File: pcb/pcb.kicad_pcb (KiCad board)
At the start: 2 copper layers, 185.3 x 78.2 mm, 22 parts, among them J1 USB_C_Receptacle, J2 Conn_01x10_Pin, J3 Conn_01x10_Pin, J4 Conn_01x10_Pin, J5 Conn_01x10_Pin, J6 Conn_01x02_Pin, SW1 SW_Push, U1 W65C02SxP, U10 74HC04, U2 W65C22SxP, U3 W65C22SxP, U4 28C256, U5 HM62256BLP, U6 74HC684, U7 74HC680, U8 74HC680, U9 74HC00, Y1 MCO-1510A

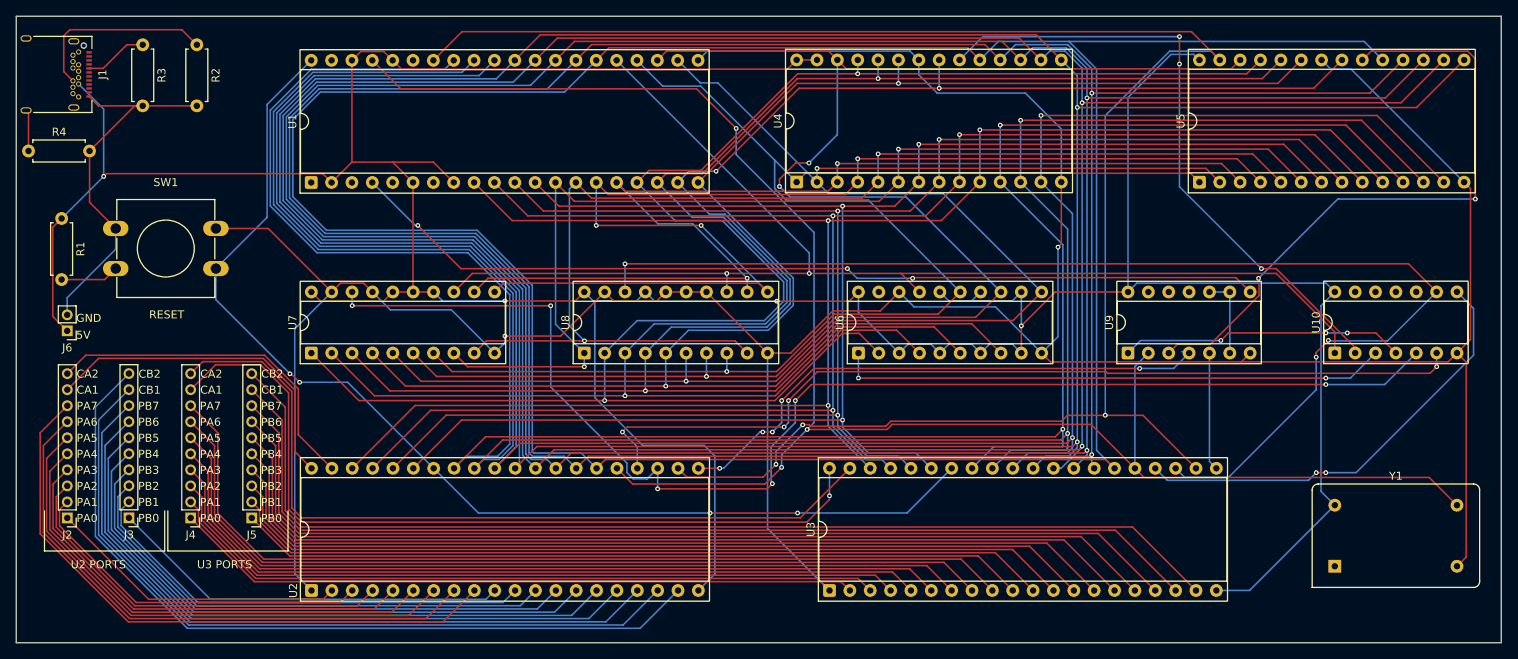
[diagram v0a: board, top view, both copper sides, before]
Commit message: update
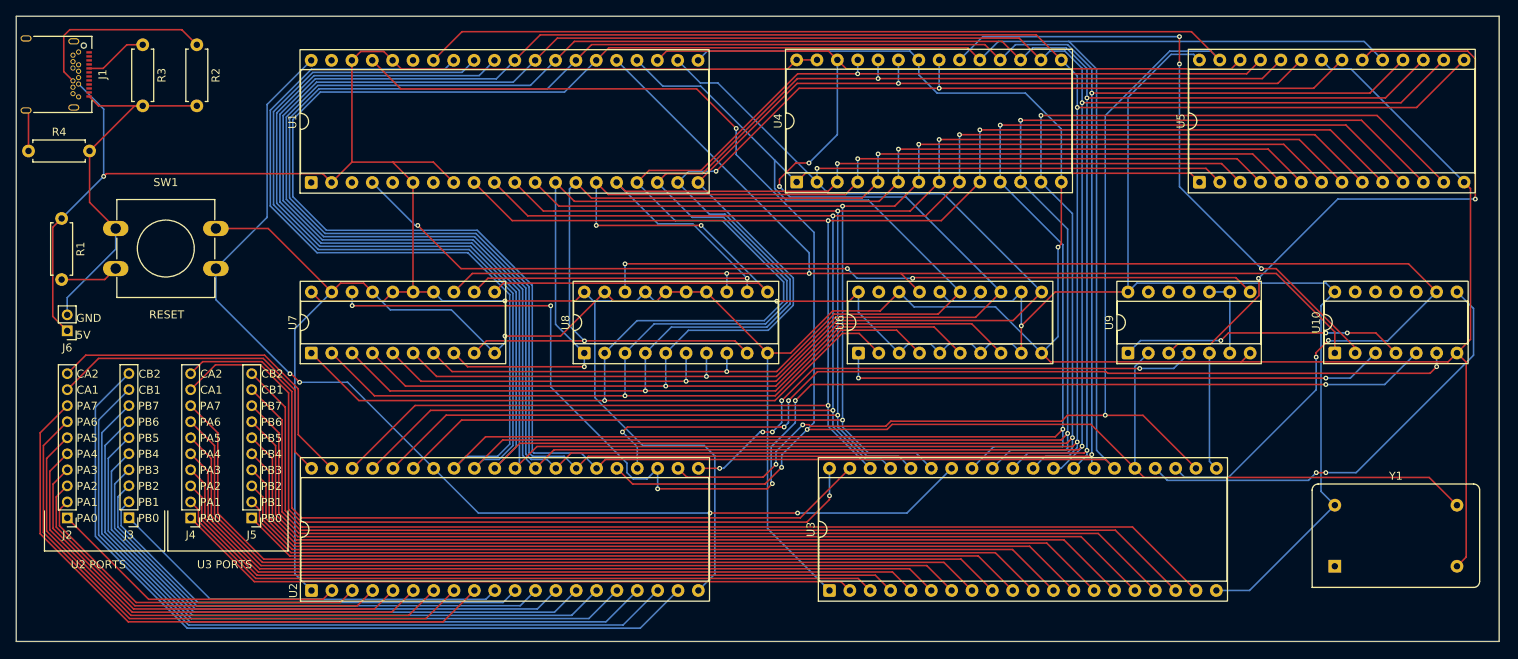
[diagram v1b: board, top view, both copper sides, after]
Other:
- board size 185.3 x 78.2 mm -> 185 x 78 mm
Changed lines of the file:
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@@
 			(drillshape 0)
 			(scaleselection 1)
-			(outputdirectory "")
+			(outputdirectory "Fabrication/")
 		)
 	)
@@
 	(gr_rect
 		(start 62.48 29.04)
-		(end 247.75 107.2)
+		(end 247.48 107.04)
 		(stroke
 			(width 0.05)

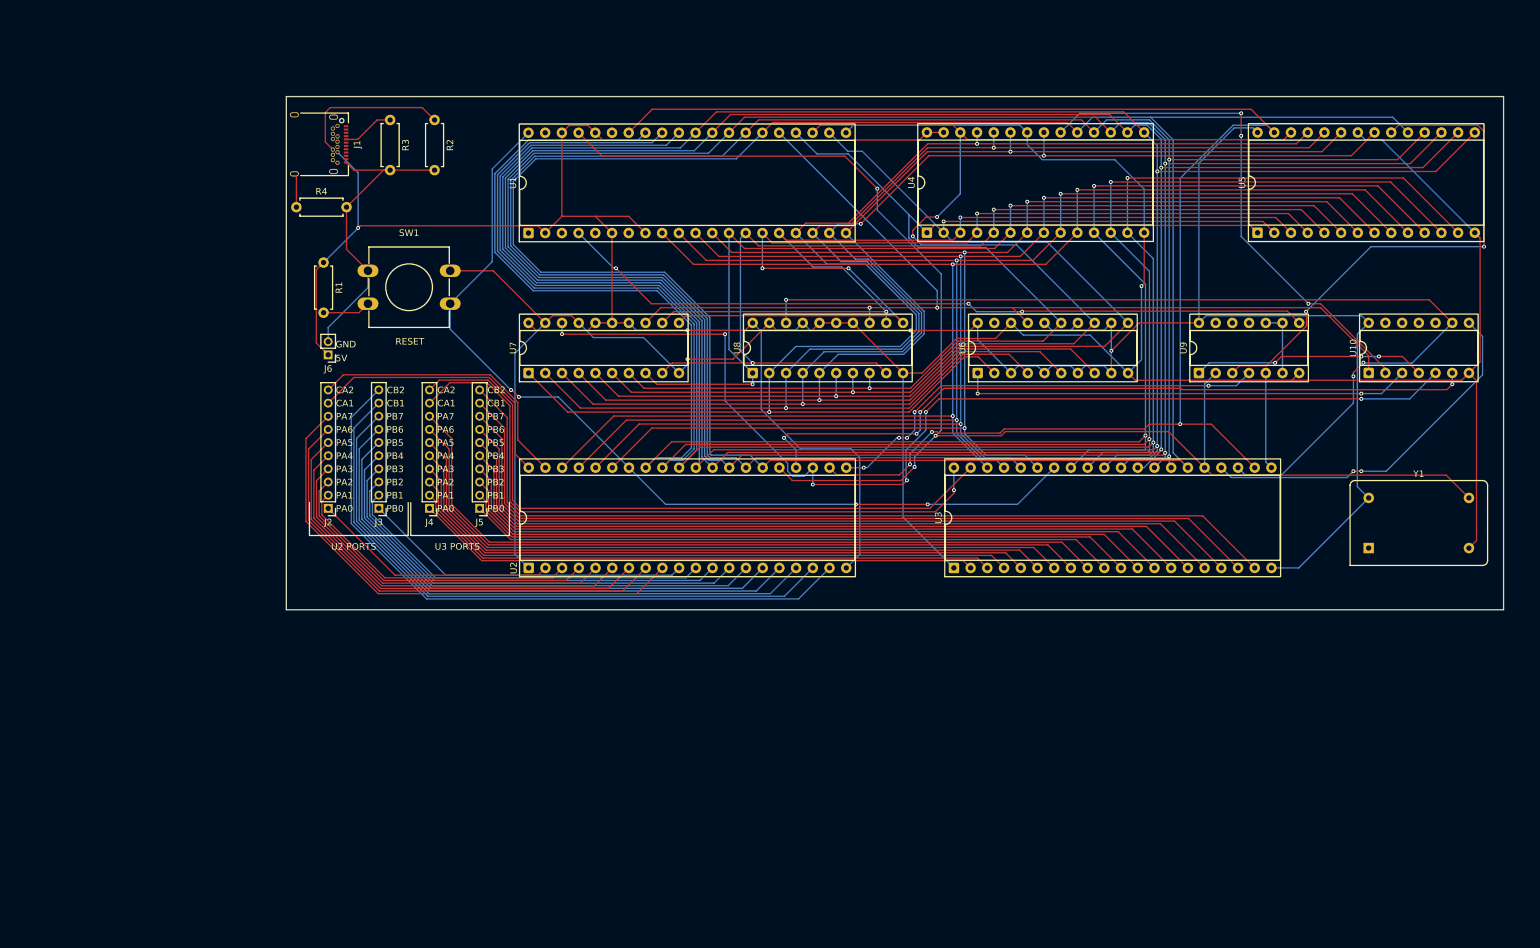
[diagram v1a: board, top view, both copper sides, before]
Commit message: Finished vesrsion 1 of the project
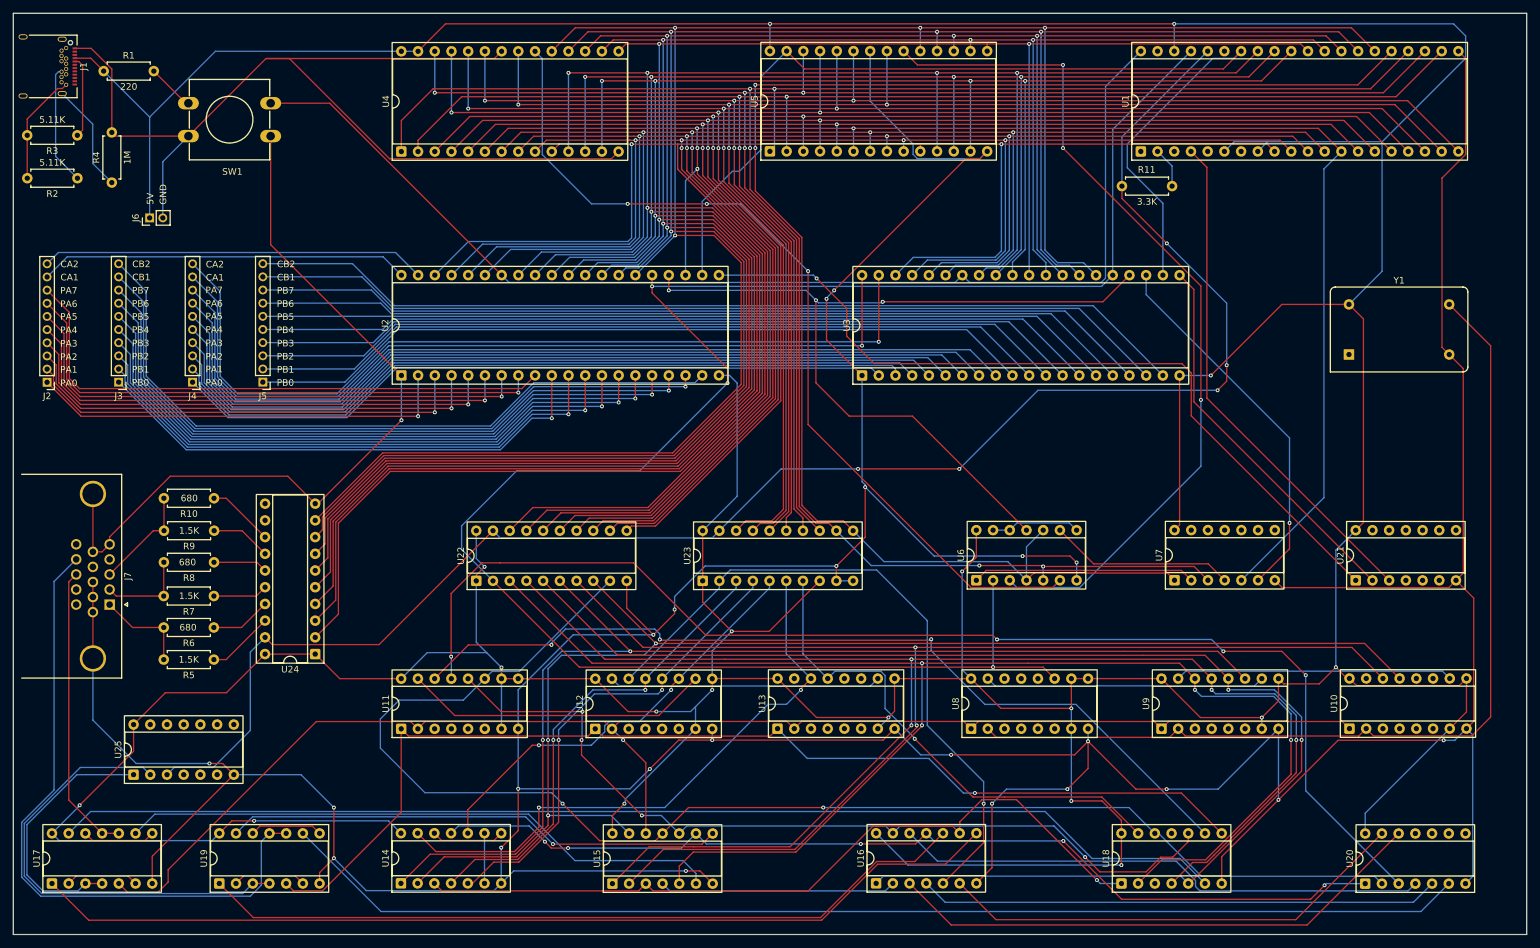
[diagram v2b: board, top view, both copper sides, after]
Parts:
- added J7: DE15_Socket_HighDensity_MountingHoles, Connector_Dsub:DSUB-15-HD_Socket_Horizontal_P2.29x2.54mm_EdgePinOffset8.35mm_Housed_MountingHolesOffset10.89mm, F.Cu at (35.6, 106.2)
- added R10: 680, Resistor_THT:R_Axial_DIN0207_L6.3mm_D2.5mm_P7.62mm_Horizontal, F.Cu at (51.5, 90.1)
- added R11: 3.3K, Resistor_THT:R_Axial_DIN0207_L6.3mm_D2.5mm_P7.62mm_Horizontal, F.Cu at (189.5, 42.6)
- added R5: 1.5K, Resistor_THT:R_Axial_DIN0207_L6.3mm_D2.5mm_P7.62mm_Horizontal, F.Cu at (51.5, 114.6)
- added R6: 680, Resistor_THT:R_Axial_DIN0207_L6.3mm_D2.5mm_P7.62mm_Horizontal, F.Cu at (51.5, 109.7)
- added R7: 1.5K, Resistor_THT:R_Axial_DIN0207_L6.3mm_D2.5mm_P7.62mm_Horizontal, F.Cu at (51.5, 105.0)
- added R8: 680, Resistor_THT:R_Axial_DIN0207_L6.3mm_D2.5mm_P7.62mm_Horizontal, F.Cu at (51.5, 99.8)
- added R9: 1.5K, Resistor_THT:R_Axial_DIN0207_L6.3mm_D2.5mm_P7.62mm_Horizontal, F.Cu at (51.5, 95.0)
- added U11: 74HC161, Package_DIP:DIP-16_W7.62mm_Socket, F.Cu at (79.9, 125.1)
- added U12: 74HC161, Package_DIP:DIP-16_W7.62mm_Socket, F.Cu at (109.4, 125.1)
- added U13: 74HC161, Package_DIP:DIP-16_W7.62mm_Socket, F.Cu at (137.1, 125.1)
- added U14: 74LS08, Package_DIP:DIP-14_W7.62mm_Socket, F.Cu at (79.9, 148.6)
- added U15: 74LS10, Package_DIP:DIP-14_W7.62mm_Socket, F.Cu at (112.0, 148.7)
- added U16: 74LS04, Package_DIP:DIP-14_W7.62mm_Socket, F.Cu at (152.1, 148.6)
- added U17: 74LS00, Package_DIP:DIP-14_W7.62mm_Socket, F.Cu at (26.9, 148.6)
- added U18: 74LS20, Package_DIP:DIP-14_W7.62mm_Socket, F.Cu at (189.4, 148.6)
- added U19: 74LS00, Package_DIP:DIP-14_W7.62mm_Socket, F.Cu at (52.3, 148.6)
- added U20: 74LS10, Package_DIP:DIP-14_W7.62mm_Socket, F.Cu at (226.4, 148.7)
- added U21: 74LS08, Package_DIP:DIP-14_W7.62mm_Socket, F.Cu at (225.0, 102.6)
- added U22: 74LS245, Package_DIP:DIP-20_W7.62mm_Socket, F.Cu at (91.3, 102.6)
- added U23: 74LS245, Package_DIP:DIP-20_W7.62mm_Socket, F.Cu at (125.8, 102.6)
- added U24: 74LS245, Package_DIP:DIP-20_W7.62mm_Socket, F.Cu at (66.9, 113.8)
- added U25: 74LS32, Package_DIP:DIP-14_W7.62mm_Socket, F.Cu at (39.3, 132.1)
- U10: value 74HC04 -> 74HC161; footprint Package_DIP:DIP-14_W7.62mm_Socket -> Package_DIP:DIP-16_W7.62mm_Socket
- U6: value 74HC684 -> 74HC00; footprint Package_DIP:DIP-20_W7.62mm_Socket -> Package_DIP:DIP-14_W7.62mm_Socket
- U7: value 74HC680 -> 74HC04; footprint Package_DIP:DIP-20_W7.62mm_Socket -> Package_DIP:DIP-14_W7.62mm_Socket
- U8: value 74HC680 -> 74HC161; footprint Package_DIP:DIP-20_W7.62mm_Socket -> Package_DIP:DIP-16_W7.62mm_Socket
- U9: value 74HC00 -> 74HC161; footprint Package_DIP:DIP-14_W7.62mm_Socket -> Package_DIP:DIP-16_W7.62mm_Socket
- Y1: value MCO-1510A -> 25.175 Mhz
- moved U7 103.1 mm to (197.5, 102.5)
- moved U1 93.9 mm to (192.3, 37.4)
- moved U4 80.8 mm to (80.0, 37.4)
- moved U5 75.1 mm to (136.0, 37.4)
- moved U8 63.4 mm to (166.6, 125.1)
- moved R2 55.0 mm to (30.7, 41.5), turned to 180 degrees
- moved U9 54.4 mm to (195.5, 125.1)
- moved U10 54.1 mm to (224.1, 125.1)
- moved R3 47.6 mm to (30.7, 34.9), turned to 180 degrees
- moved J2 46.8 mm to (26.1, 72.5)
- moved R1 44.3 mm to (34.7, 25.2), turned to 0 degrees
- moved J3 43.9 mm to (37.0, 72.5)
- moved J1 42.9 mm to (25.3, 24.5)
- moved J4 40.8 mm to (48.2, 72.5)
- moved J5 38.1 mm to (58.9, 72.4)
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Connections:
- U1 pad 13: /A4 -> ~{CS}_{VIA A}
- U1 pad 2: +5V -> Net-(U1-RDY)
- U1 pad 36: +5V -> CPU/~{VGA}
- U1 pad 37: CLK -> Clock
- U10 pad 1: /A15 -> Net-(U10-~{MR})
- U10 pad 10: (no net) -> Net-(U10-CET)
- U10 pad 11: (no net) -> unconnected-(U10-Q3-Pad11)
- U10 pad 12: (no net) -> unconnected-(U10-Q2-Pad12)
- U10 pad 13: (no net) -> /Q9A
- U10 pad 14: +5V -> /Q8A
- U10 pad 2: Net-(U4-~{CS}) -> Net-(U10-CP)
- U10 pad 3: Net-(U6-~{P>Q}) -> unconnected-(U10-D0-Pad3)
- U10 pad 4: Net-(U10-Pad4) -> unconnected-(U10-D1-Pad4)
- U10 pad 5: Net-(U2-~{CS2}) -> unconnected-(U10-D2-Pad5)
- U10 pad 6: Net-(U2-CS1) -> unconnected-(U10-D3-Pad6)
- U10 pad 7: GND -> +5V
- U10 pad 8: Net-(U3-CS1) -> GND
- U10 pad 9: Net-(U3-~{CS2}) -> +5V
- U2 pad 23: Net-(U2-~{CS2}) -> ~{CS}_{VIA A}
- U2 pad 24: Net-(U2-CS1) -> VIA Enable
- U2 pad 25: CLK -> Clock
- U3 pad 23: Net-(U3-~{CS2}) -> ~{CS}_{VIA B}
- U3 pad 24: Net-(U3-CS1) -> VIA Enable
- U3 pad 25: CLK -> Clock
- U4 pad 20: Net-(U4-~{CS}) -> ~{CS}_{ROM}
- U4 pad 6: /A4 -> ~{CS}_{VIA A}
- U5 pad 20: Net-(U5-~{CS}) -> ~{CS}_{RAM}
- U5 pad 6: /A4 -> ~{CS}_{VIA A}
- U6 pad 1: Net-(U6-~{P>Q}) -> Net-(U6-Pad1)
- U6 pad 10: GND -> /A15
- U6 pad 11: /A12 -> VIA Enable
- U6 pad 12: +5V -> Net-(U6-Pad12)
- U6 pad 13: /A13 -> Net-(U6-Pad12)
- U6 pad 2: /A8 -> Clock
- U6 pad 3: +5V -> ~{CS}_{RAM}
- U6 pad 4: /A9 -> /A15
- U6 pad 5: +5V -> /A14
- U6 pad 6: /A10 -> ~{CS}_{ROM}
- U6 pad 7: +5V -> GND
- U6 pad 8: /A11 -> Net-(U6-Pad12)
- U6 pad 9: +5V -> Net-(U6-Pad9)
- U7 pad 1: /A8 -> /A15
- U7 pad 10: GND -> (no net)
- U7 pad 11: /A6 -> (no net)
- U7 pad 12: /A7 -> (no net)
- U7 pad 13: /A15 -> (no net)
- U7 pad 2: /A9 -> Net-(U6-Pad1)
- U7 pad 3: /A10 -> /A14
- U7 pad 4: /A11 -> Net-(U6-Pad9)
- U7 pad 5: /A12 -> ~{CS}_{VIA A}
- U7 pad 6: /A13 -> ~{CS}_{VIA B}
- U7 pad 7: /A14 -> GND
- U7 pad 8: /A4 -> (no net)
- U7 pad 9: /A5 -> (no net)
- U8 pad 1: /A4 -> Net-(U10-~{MR})
- U8 pad 10: GND -> +5V
- U8 pad 11: /A6 -> Clock
- U8 pad 12: /A7 -> unconnected-(U8-Q2-Pad12)
- U8 pad 13: /A15 -> unconnected-(U8-Q1-Pad13)
- U8 pad 14: GND -> unconnected-(U8-Q0-Pad14)
- U8 pad 15: GND -> Net-(U8-TC)
- U8 pad 16: GND -> +5V
- U8 pad 2: /A8 -> Net-(U10-CP)
- U8 pad 3: /A9 -> unconnected-(U8-D0-Pad3)
- U8 pad 4: /A10 -> unconnected-(U8-D1-Pad4)
- U8 pad 5: /A11 -> unconnected-(U8-D2-Pad5)
- U8 pad 6: /A12 -> unconnected-(U8-D3-Pad6)
- U8 pad 7: /A13 -> +5V
- U8 pad 8: /A14 -> GND
- U8 pad 9: /A5 -> +5V
- U9 pad 1: Net-(U10-Pad4) -> Net-(U10-~{MR})
- U9 pad 10: Net-(U9-Pad10) -> Net-(U8-TC)
- U9 pad 11: (no net) -> /Q7A
- U9 pad 12: (no net) -> /Q6A
- U9 pad 13: (no net) -> /Q5A
- U9 pad 14: +5V -> /Q4A
- U9 pad 2: CLK -> Net-(U10-CP)
- U9 pad 3: Net-(U5-~{CS}) -> unconnected-(U9-D0-Pad3)
- U9 pad 4: ~{IRQ} 1 -> unconnected-(U9-D1-Pad4)
- U9 pad 5: ~{IRQ} 2 -> unconnected-(U9-D2-Pad5)
- U9 pad 6: Net-(U9-Pad10) -> unconnected-(U9-D3-Pad6)
- U9 pad 7: GND -> +5V
- U9 pad 8: Net-(U1-~{IRQ}) -> GND
- U9 pad 9: Net-(U9-Pad10) -> +5V
- Y1 pad 8: CLK -> Net-(U10-CP)
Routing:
- net GND: track 452.8 -> 1090.3 mm, vias 2 -> 24
- net +5V: track 463.9 -> 1000.6 mm, vias 4 -> 18
- net ~{CS}_{VIA A}: track 0.00 -> 308.9 mm, vias 0 -> 4
- net Clock: track 0.00 -> 295.3 mm, vias 0 -> 3
- net CPU/~{VGA}: track 0.00 -> 256.8 mm, vias 0 -> 5
- net /Q5A: track 0.00 -> 226.6 mm, vias 0 -> 4
- net /Q4A: track 0.00 -> 225.2 mm, vias 0 -> 4
- net Net-(U10-~{MR}): track 0.00 -> 222.5 mm, vias 0 -> 1
- net CLK: track 219.7 -> 0.00 mm, vias 3 -> 0
- net /Q3B: track 0.00 -> 212.9 mm, vias 0 -> 2
- net /Q9A: track 0.00 -> 207.4 mm, vias 0 -> 3
- net /Q6A: track 0.00 -> 205.7 mm, vias 0 -> 2
- net /Q8A: track 0.00 -> 194.5 mm, vias 0 -> 2
- net /Q1B: track 0.00 -> 189.4 mm, vias 0 -> 4
- net Net-(U19-Pad9): track 0.00 -> 180.8 mm
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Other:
- board size 185 x 78 mm -> 230 x 140 mm
- board text removed: "RESET"
- board text removed: "U2 PORTS"
- board text removed: "U3 PORTS"

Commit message: started working on version 2.0
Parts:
- removed J4, J5: Conn_01x10_Pin, Connector_PinHeader_2.00mm:PinHeader_1x10_P2.00mm_Vertical
- removed J6: Conn_01x02_Pin, Connector_PinHeader_2.00mm:PinHeader_1x02_P2.00mm_Vertical
- removed J7: DE15_Socket_HighDensity_MountingHoles, Connector_Dsub:DSUB-15-HD_Socket_Horizontal_P2.29x2.54mm_EdgePinOffset8.35mm_Housed_MountingHolesOffset10.89mm
- removed R10, R8: 680, Resistor_THT:R_Axial_DIN0207_L6.3mm_D2.5mm_P7.62mm_Horizontal
- removed R11: 3.3K, Resistor_THT:R_Axial_DIN0207_L6.3mm_D2.5mm_P7.62mm_Horizontal
- removed R9: 1.5K, Resistor_THT:R_Axial_DIN0207_L6.3mm_D2.5mm_P7.62mm_Horizontal
- removed U10, U11, U12, U13: 74HC161, Package_DIP:DIP-16_W7.62mm_Socket
- removed U14, U21: 74LS08, Package_DIP:DIP-14_W7.62mm_Socket
- removed U15, U20: 74LS10, Package_DIP:DIP-14_W7.62mm_Socket
- removed U16: 74LS04, Package_DIP:DIP-14_W7.62mm_Socket
- removed U17, U19: 74LS00, Package_DIP:DIP-14_W7.62mm_Socket
- removed U18: 74LS20, Package_DIP:DIP-14_W7.62mm_Socket
- removed U22, U23, U24: 74LS245, Package_DIP:DIP-20_W7.62mm_Socket
- removed U25: 74LS32, Package_DIP:DIP-14_W7.62mm_Socket
- removed Y1: 25.175 Mhz, Oscillator:Oscillator_DIP-14
- added C1: 100nF, Capacitor_SMD:C_0805_2012Metric_Pad1.18x1.45mm_HandSolder, B.Cu at (87.1, 47.8)
- added C2: 100nF, Capacitor_SMD:C_0805_2012Metric_Pad1.18x1.45mm_HandSolder, B.Cu at (169.8, 33.9)
- added C3: 100nF, Capacitor_SMD:C_0805_2012Metric_Pad1.18x1.45mm_HandSolder, B.Cu at (125.3, 37.6)
- added C4: 100nF, Capacitor_SMD:C_0805_2012Metric_Pad1.18x1.45mm_HandSolder, F.Cu at (117.8, 79.1)
- added C5: 100nF, Capacitor_SMD:C_0805_2012Metric_Pad1.18x1.45mm_HandSolder, F.Cu at (172.2, 79.1)
- added C6: 100nF, Capacitor_SMD:C_0805_2012Metric_Pad1.18x1.45mm_HandSolder, B.Cu at (56.0, 39.0)
- added C7: 100nF, Capacitor_SMD:C_0805_2012Metric_Pad1.18x1.45mm_HandSolder, F.Cu at (62.0, 32.8)
- J2, J3: value Conn_01x10_Pin -> 2x20 Header; footprint Connector_PinHeader_2.00mm:PinHeader_1x10_P2.00mm_Vertical -> Connector_PinHeader_2.54mm:PinHeader_2x10_P2.54mm_Vertical
- R1: value 220 -> 1M; footprint Resistor_THT:R_Axial_DIN0207_L6.3mm_D2.5mm_P7.62mm_Horizontal -> Resistor_SMD:R_0805_2012Metric_Pad1.20x1.40mm_HandSolder
- R2, R3: value 5.11K -> 5K1; footprint Resistor_THT:R_Axial_DIN0207_L6.3mm_D2.5mm_P7.62mm_Horizontal -> Resistor_SMD:R_0805_2012Metric_Pad1.20x1.40mm_HandSolder
- R4: value 1M -> 3K3; footprint Resistor_THT:R_Axial_DIN0207_L6.3mm_D2.5mm_P7.62mm_Horizontal -> Resistor_SMD:R_0805_2012Metric_Pad1.20x1.40mm_HandSolder; moved to B.Cu
- R5: value 1.5K -> 10K; footprint Resistor_THT:R_Axial_DIN0207_L6.3mm_D2.5mm_P7.62mm_Horizontal -> Resistor_SMD:R_0805_2012Metric_Pad1.20x1.40mm_HandSolder
- R6: value 680 -> 1M; footprint Resistor_THT:R_Axial_DIN0207_L6.3mm_D2.5mm_P7.62mm_Horizontal -> Resistor_SMD:R_0805_2012Metric_Pad1.20x1.40mm_HandSolder
- R7: value 1.5K -> 10K; footprint Resistor_THT:R_Axial_DIN0207_L6.3mm_D2.5mm_P7.62mm_Horizontal -> Resistor_SMD:R_0805_2012Metric_Pad1.20x1.40mm_HandSolder; moved to B.Cu
- SW1: footprint Button_Switch_THT:SW_PUSH-12mm -> Button_Switch_THT:SW_TH_Tactile_Omron_B3F-100x
- U1: value W65C02SxP -> W65C02
- U2: value W65C22SxP -> 28C256; footprint Package_DIP:DIP-40_W15.24mm_Socket -> Socket:DIP_Socket-28_W11.9mm_W12.7mm_W15.24mm_W17.78mm_W18.5mm_3M_228-1277-00-0602J
- U3: value W65C22SxP -> 62256; footprint Package_DIP:DIP-40_W15.24mm_Socket -> Package_DIP:DIP-28_W15.24mm_Socket
- U4: value 28C256 -> W65C22S; footprint Package_DIP:DIP-28_W15.24mm_Socket -> Package_DIP:DIP-40_W15.24mm_Socket
- U5: value HM62256BLP -> W65C22S; footprint Package_DIP:DIP-28_W15.24mm_Socket -> Package_DIP:DIP-40_W15.24mm_Socket
- U6: value 74HC00 -> 74AC00
- U7: value 74HC04 -> 74LS04
- U8: value 74HC161 -> 74LS08; footprint Package_DIP:DIP-16_W7.62mm_Socket -> Package_DIP:DIP-14_W7.62mm_Socket
- U9: value 74HC161 -> 555; footprint Package_DIP:DIP-16_W7.62mm_Socket -> Package_DIP:DIP-8_W7.62mm
- moved U7 336.3 mm to (-132.4, 37.0), turned to 0 degrees
- moved U6 318.3 mm to (-144.1, 37.0), turned to 0 degrees
- moved U8 300.5 mm to (-120.7, 37.0), turned to 0 degrees
- moved U9 162.0 mm to (56.0, 42.8)
- moved U2 126.8 mm to (201.8, 36.4), turned to -90 degrees
- moved U1 122.7 mm to (70.3, 50.3)
- moved R5 82.7 mm to (42.0, 32.5), turned to -90 degrees
- moved R6 77.2 mm to (57.0, 32.8), turned to 0 degrees
- moved R7 64.8 mm to (82.0, 47.8), turned to 0 degrees
- moved U5 40.0 mm to (124.9, 75.8)
- moved U4 39.6 mm to (70.5, 75.8)
- moved R4 36.9 mm to (72.9, 42.7), turned to -90 degrees
- moved U3 33.2 mm to (124.3, 50.3)
- moved J3 25.0 mm to (52.8, 53.0), turned to 0 degrees
- moved J2 21.9 mm to (36.1, 53.0), turned to 0 degrees
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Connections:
- J2 pad 1: Net-(J2-Pin_1) -> Net-(U4-PA0)
- J2 pad 10: Net-(J2-Pin_10) -> Net-(U4-PB4)
- J2 pad 2: Net-(J2-Pin_2) -> Net-(U4-PB0)
- J2 pad 3: Net-(J2-Pin_3) -> Net-(U4-PA1)
- J2 pad 4: Net-(J2-Pin_4) -> Net-(U4-PB1)
- J2 pad 5: Net-(J2-Pin_5) -> Net-(U4-PA2)
- J2 pad 6: Net-(J2-Pin_6) -> Net-(U4-PB2)
- J2 pad 7: Net-(J2-Pin_7) -> Net-(U4-PA3)
- J2 pad 8: Net-(J2-Pin_8) -> Net-(U4-PB3)
- J2 pad 9: Net-(J2-Pin_9) -> Net-(U4-PA4)
- J3 pad 1: Net-(J3-Pin_1) -> Net-(U5-PA0)
- J3 pad 10: Net-(J3-Pin_10) -> Net-(U5-PB4)
- J3 pad 2: Net-(J3-Pin_2) -> Net-(U5-PB0)
- J3 pad 3: Net-(J3-Pin_3) -> Net-(U5-PA1)
- J3 pad 4: Net-(J3-Pin_4) -> Net-(U5-PB1)
- J3 pad 5: Net-(J3-Pin_5) -> Net-(U5-PA2)
- J3 pad 6: Net-(J3-Pin_6) -> Net-(U5-PB2)
- J3 pad 7: Net-(J3-Pin_7) -> Net-(U5-PA3)
- J3 pad 8: Net-(J3-Pin_8) -> Net-(U5-PB3)
- J3 pad 9: Net-(J3-Pin_9) -> Net-(U5-PA4)
- R1 pad 1: +5V -> Net-(J1-SHIELD)
- R1 pad 2: ~{RES} -> GND
- R4 pad 1: Net-(J1-SHIELD) -> Net-(U1-BE)
- R4 pad 2: GND -> Net-(U1-RDY)
- R5 pad 1: Net-(U24-B0) -> +5V
- R5 pad 2: Net-(J7-Pad1) -> Net-(U9-TR)
- R6 pad 1: Net-(U24-B1) -> +5V
- R6 pad 2: Net-(J7-Pad1) -> Net-(U9-DIS)
- R7 pad 1: Net-(U24-B2) -> +5V
- R7 pad 2: Net-(J7-Pad2) -> ~{NMI}
- SW1 pad 2: ~{RES} -> Net-(U9-TR)
- U1 pad 13: ~{CS}_{VIA A} -> /A4
- U1 pad 36: CPU/~{VGA} -> Net-(U1-BE)
- U1 pad 37: Clock -> CLK
- U1 pad 4: Net-(U1-~{IRQ}) -> ~{IRQ}
- U1 pad 6: +5V -> ~{NMI}
- U2 pad 1: GND -> /A14
- U2 pad 10: Net-(J3-Pin_1) -> /A0
- U2 pad 11: Net-(J3-Pin_2) -> /D0
- U2 pad 12: Net-(J3-Pin_3) -> /D1
- U2 pad 13: Net-(J3-Pin_4) -> /D2
- U2 pad 14: Net-(J3-Pin_5) -> GND
- U2 pad 15: Net-(J3-Pin_6) -> /D3
- U2 pad 16: Net-(J3-Pin_7) -> /D4
- U2 pad 17: Net-(J3-Pin_8) -> /D5
- U2 pad 18: Net-(J3-Pin_9) -> /D6
- U2 pad 19: Net-(J3-Pin_10) -> /D7
- U2 pad 2: Net-(J2-Pin_1) -> /A12
- U2 pad 20: +5V -> unconnected-(U2-~{CS}-Pad20)
- U2 pad 21: ~{IRQ} 1 -> /A10
- U2 pad 22: R/~{W} -> GND
- U2 pad 23: ~{CS}_{VIA A} -> /A11
- U2 pad 24: VIA Enable -> /A9
- U2 pad 25: Clock -> /A8
- U2 pad 26: /D7 -> /A13
- U2 pad 27: /D6 -> GND
- U2 pad 28: /D5 -> +5V
- U2 pad 3: Net-(J2-Pin_2) -> /A7
- U2 pad 4: Net-(J2-Pin_3) -> /A6
- U2 pad 5: Net-(J2-Pin_4) -> /A5
- U2 pad 6: Net-(J2-Pin_5) -> /A4
- U2 pad 7: Net-(J2-Pin_6) -> /A3
- U2 pad 8: Net-(J2-Pin_7) -> /A2
- U2 pad 9: Net-(J2-Pin_8) -> /A1
- U3 pad 1: GND -> /A14
- U3 pad 10: Net-(J5-Pin_1) -> /A0
- U3 pad 11: Net-(J5-Pin_2) -> /D0
- U3 pad 12: Net-(J5-Pin_3) -> /D1
- U3 pad 13: Net-(J5-Pin_4) -> /D2
- U3 pad 14: Net-(J5-Pin_5) -> GND
- U3 pad 15: Net-(J5-Pin_6) -> /D3
- U3 pad 16: Net-(J5-Pin_7) -> /D4
- U3 pad 17: Net-(J5-Pin_8) -> /D5
- U3 pad 18: Net-(J5-Pin_9) -> /D6
- U3 pad 19: Net-(J5-Pin_10) -> /D7
- U3 pad 2: Net-(J4-Pin_1) -> /A12
- U3 pad 20: +5V -> unconnected-(U3-~{CS}-Pad20)
- U3 pad 21: ~{IRQ} 2 -> /A10
- U3 pad 22: R/~{W} -> GND
- U3 pad 23: ~{CS}_{VIA B} -> /A11
- U3 pad 24: VIA Enable -> /A9
- U3 pad 25: Clock -> /A8
- U3 pad 26: /D7 -> /A13
- U3 pad 27: /D6 -> R/~{W}
- U3 pad 28: /D5 -> +5V
- U3 pad 3: Net-(J4-Pin_2) -> /A7
- U3 pad 4: Net-(J4-Pin_3) -> /A6
- U3 pad 5: Net-(J4-Pin_4) -> /A5
- U3 pad 6: Net-(J4-Pin_5) -> /A4
- U3 pad 7: Net-(J4-Pin_6) -> /A3
- U3 pad 8: Net-(J4-Pin_7) -> /A2
- U3 pad 9: Net-(J4-Pin_8) -> /A1
- U4 pad 1: /A14 -> GND
- U4 pad 10: /A0 -> Net-(U4-PB0)
- U4 pad 11: /D0 -> Net-(U4-PB1)
- U4 pad 12: /D1 -> Net-(U4-PB2)
- U4 pad 13: /D2 -> Net-(U4-PB3)
- U4 pad 14: GND -> Net-(U4-PB4)
- U4 pad 15: /D3 -> Net-(U4-PB5)
- U4 pad 16: /D4 -> Net-(U4-PB6)
- U4 pad 17: /D5 -> Net-(U4-PB7)
- U4 pad 18: /D6 -> Net-(U4-CB1)
- U4 pad 19: /D7 -> Net-(U4-CB2)
- U4 pad 2: /A12 -> Net-(U4-PA0)
- U4 pad 20: ~{CS}_{ROM} -> +5V
- U4 pad 21: /A10 -> ~{IRQ} 2
- U4 pad 22: GND -> unconnected-(U4-R/~{W}-Pad22)
- U4 pad 23: /A11 -> unconnected-(U4-~{CS2}-Pad23)
- U4 pad 24: /A9 -> unconnected-(U4-CS1-Pad24)
- U4 pad 25: /A8 -> unconnected-(U4-ϕ2-Pad25)
- U4 pad 26: /A13 -> /D7
- U4 pad 27: +5V -> /D6
- U4 pad 28: +5V -> /D5
- U4 pad 3: /A7 -> Net-(U4-PA1)
- U4 pad 4: /A6 -> Net-(U4-PA2)
- U4 pad 5: /A5 -> Net-(U4-PA3)
- U4 pad 6: ~{CS}_{VIA A} -> Net-(U4-PA4)
- U4 pad 7: /A3 -> Net-(U4-PA5)
- U4 pad 8: /A2 -> Net-(U4-PA6)
- U4 pad 9: /A1 -> Net-(U4-PA7)
- U5 pad 1: /A14 -> GND
- U5 pad 10: /A0 -> Net-(U5-PB0)
- U5 pad 11: /D0 -> Net-(U5-PB1)
- U5 pad 12: /D1 -> Net-(U5-PB2)
- U5 pad 13: /D2 -> Net-(U5-PB3)
- U5 pad 14: GND -> Net-(U5-PB4)
- U5 pad 15: /D3 -> Net-(U5-PB5)
- U5 pad 16: /D4 -> Net-(U5-PB6)
- U5 pad 17: /D5 -> Net-(U5-PB7)
- U5 pad 18: /D6 -> Net-(U5-CB1)
- U5 pad 19: /D7 -> Net-(U5-CB2)
- U5 pad 2: /A12 -> Net-(U5-PA0)
- U5 pad 20: ~{CS}_{RAM} -> +5V
- U5 pad 21: /A10 -> ~{IRQ} 1
- U5 pad 22: GND -> unconnected-(U5-R/~{W}-Pad22)
- U5 pad 23: /A11 -> unconnected-(U5-~{CS2}-Pad23)
- U5 pad 24: /A9 -> unconnected-(U5-CS1-Pad24)
- U5 pad 25: /A8 -> unconnected-(U5-ϕ2-Pad25)
- U5 pad 26: /A13 -> /D7
- U5 pad 27: R/~{W} -> /D6
- U5 pad 28: +5V -> /D5
- U5 pad 3: /A7 -> Net-(U5-PA1)
- U5 pad 4: /A6 -> Net-(U5-PA2)
- U5 pad 5: /A5 -> Net-(U5-PA3)
- U5 pad 6: ~{CS}_{VIA A} -> Net-(U5-PA4)
- U5 pad 7: /A3 -> Net-(U5-PA5)
- U5 pad 8: /A2 -> Net-(U5-PA6)
- U5 pad 9: /A1 -> Net-(U5-PA7)
- U6 pad 1: Net-(U6-Pad1) -> unconnected-(U6-Pad1)
- U6 pad 10: /A15 -> unconnected-(U6-Pad10)
- U6 pad 11: VIA Enable -> unconnected-(U6-Pad11)
- U6 pad 12: Net-(U6-Pad12) -> unconnected-(U6-Pad12)
- U6 pad 13: Net-(U6-Pad12) -> unconnected-(U6-Pad13)
- U6 pad 14: +5V -> unconnected-(U6E-VCC-Pad14)
- U6 pad 2: Clock -> unconnected-(U6-Pad2)
- U6 pad 3: ~{CS}_{RAM} -> unconnected-(U6-Pad3)
- U6 pad 4: /A15 -> unconnected-(U6-Pad4)
- U6 pad 5: /A14 -> unconnected-(U6-Pad5)
- U6 pad 6: ~{CS}_{ROM} -> unconnected-(U6-Pad6)
- U6 pad 7: GND -> unconnected-(U6E-GND-Pad7)
- U6 pad 8: Net-(U6-Pad12) -> unconnected-(U6-Pad8)
- U6 pad 9: Net-(U6-Pad9) -> unconnected-(U6-Pad9)
- U7 pad 1: /A15 -> unconnected-(U7-Pad1)
- U7 pad 10: (no net) -> unconnected-(U7-Pad10)
- U7 pad 11: (no net) -> unconnected-(U7-Pad11)
- U7 pad 12: (no net) -> unconnected-(U7-Pad12)
- U7 pad 13: (no net) -> unconnected-(U7-Pad13)
- U7 pad 14: +5V -> unconnected-(U7G-VCC-Pad14)
- U7 pad 2: Net-(U6-Pad1) -> unconnected-(U7-Pad2)
- U7 pad 3: /A14 -> unconnected-(U7-Pad3)
- U7 pad 4: Net-(U6-Pad9) -> unconnected-(U7-Pad4)
- U7 pad 5: ~{CS}_{VIA A} -> unconnected-(U7-Pad5)
- U7 pad 6: ~{CS}_{VIA B} -> unconnected-(U7-Pad6)
- U7 pad 7: GND -> unconnected-(U7G-GND-Pad7)
- U7 pad 8: (no net) -> unconnected-(U7-Pad8)
- U7 pad 9: (no net) -> unconnected-(U7-Pad9)
- U8 pad 1: Net-(U10-~{MR}) -> unconnected-(U8-Pad1)
- U8 pad 10: +5V -> unconnected-(U8-Pad10)
- U8 pad 11: Clock -> unconnected-(U8-Pad11)
- U8 pad 2: Net-(U10-CP) -> unconnected-(U8-Pad2)
- U8 pad 7: +5V -> unconnected-(U8E-GND-Pad7)
- U8 pad 8: GND -> unconnected-(U8-Pad8)
- U8 pad 9: +5V -> unconnected-(U8-Pad9)
- U9 pad 1: Net-(U10-~{MR}) -> GND
- U9 pad 2: Net-(U10-CP) -> Net-(U9-TR)
- U9 pad 3: unconnected-(U9-D0-Pad3) -> ~{RES}
- U9 pad 6: unconnected-(U9-D3-Pad6) -> Net-(U9-DIS)
- U9 pad 7: +5V -> Net-(U9-DIS)
- U9 pad 8: GND -> +5V
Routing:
- net GND: track 1090.3 -> 0.00 mm, vias 24 -> 0
- net +5V: track 1000.6 -> 0.00 mm, vias 18 -> 0
- net /D0: track 343.2 -> 0.00 mm, vias 5 -> 0
- net /D1: track 333.1 -> 0.00 mm, vias 5 -> 0
- net /D2: track 324.1 -> 0.00 mm, vias 5 -> 0
- net /D7: track 318.4 -> 0.00 mm, vias 4 -> 0
- net /D6: track 315.0 -> 0.00 mm, vias 4 -> 0
- net /D5: track 311.6 -> 0.00 mm, vias 4 -> 0
- net /D4: track 309.4 -> 0.00 mm, vias 4 -> 0
- net ~{CS}_{VIA A}: track 308.9 -> 0.00 mm, vias 4 -> 0
- net /A14: track 307.3 -> 0.00 mm, vias 5 -> 0
- net /D3: track 307.2 -> 0.00 mm, vias 3 -> 0
- net Clock: track 295.3 -> 0.00 mm, vias 3 -> 0
- net /A3: track 288.1 -> 0.00 mm, vias 5 -> 0
- net /A2: track 286.2 -> 0.00 mm, vias 5 -> 0
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- added copper zone on In2.Cu, net +5V
- added copper zone on In1.Cu, net GND
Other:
- board size 230 x 140 mm -> 185 x 100 mm
- copper layers 2 -> 4
- board text removed: "5V"
- board text removed: "CA1"
- board text removed: "CA2"
- board text removed: "CB1"
- board text removed: "CB2"
- board text removed: "GND"
- board text removed: "PA0"
- board text removed: "PA1"
- board text removed: "PA2"
- board text removed: "PA3"
- board text removed: "PA4"
- board text removed: "PA5"
- board text removed: "PA6"
- board text removed: "PA7"
- board text removed: "PB0"
- board text removed: "PB1"
- board text removed: "PB2"
- board text removed: "PB3"
- board text removed: "PB4"
- board text removed: "PB5"
- board text removed: "PB6"
- board text removed: "PB7"
